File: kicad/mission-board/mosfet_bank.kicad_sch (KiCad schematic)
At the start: 28 parts, among them J10 MOSFET Ch2 Out, J11 MOSFET Ch3 Out, J12 MOSFET Ch4 Out, J9 MOSFET Ch1 Out, Q2 AO3400A, Q3 AO3400A, Q4 AO3400A, Q5 AO3400A, U4 INA180A2IDBVR, U5 INA180A2IDBVR, U6 INA180A2IDBVR, U7 INA180A2IDBVR

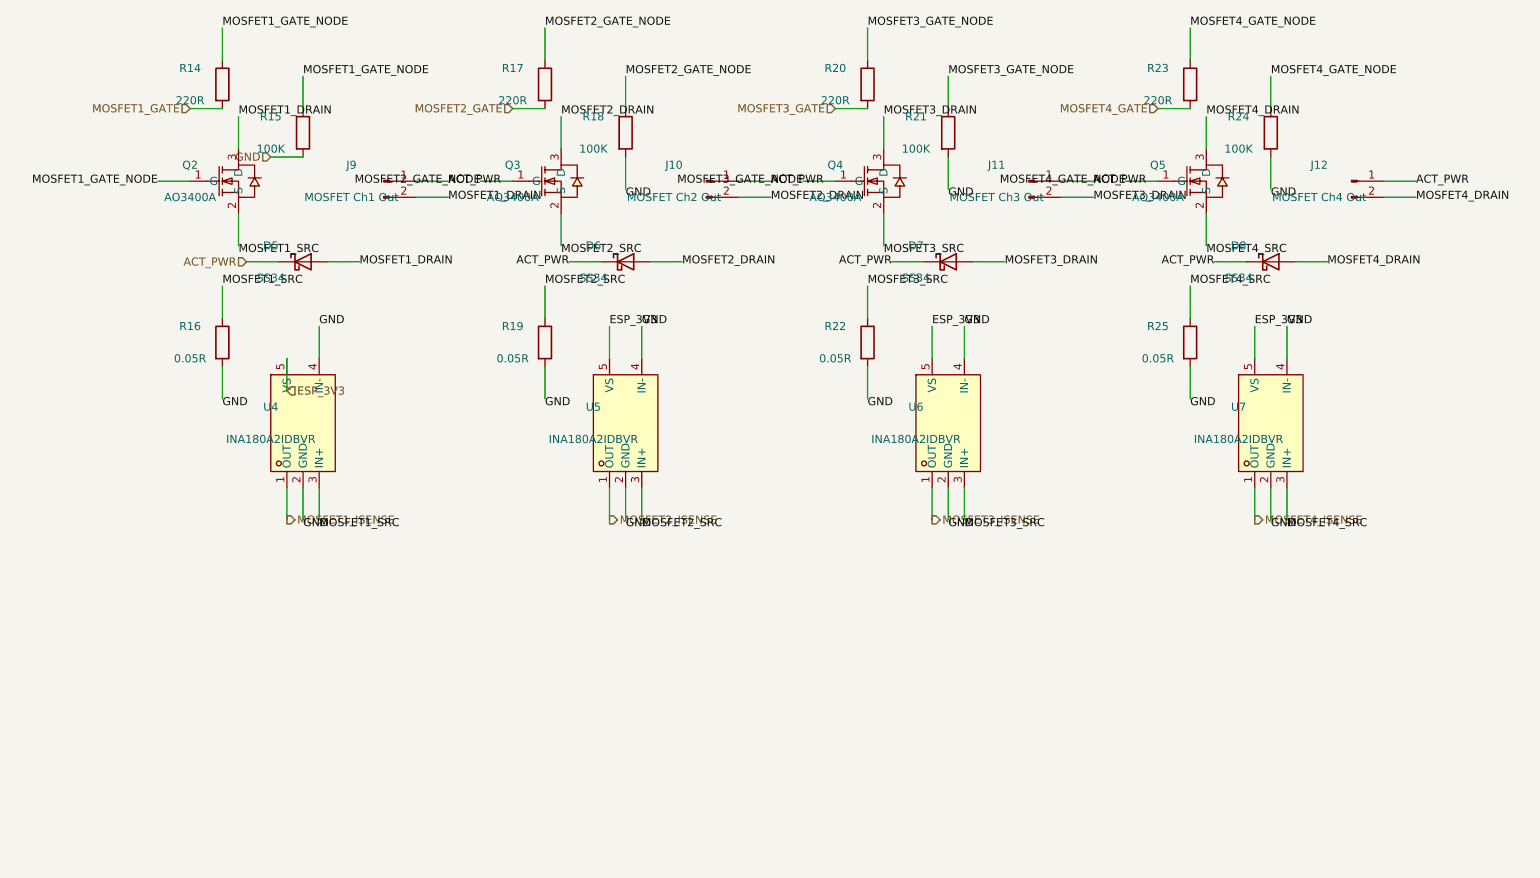
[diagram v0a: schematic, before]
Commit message: pcb progress
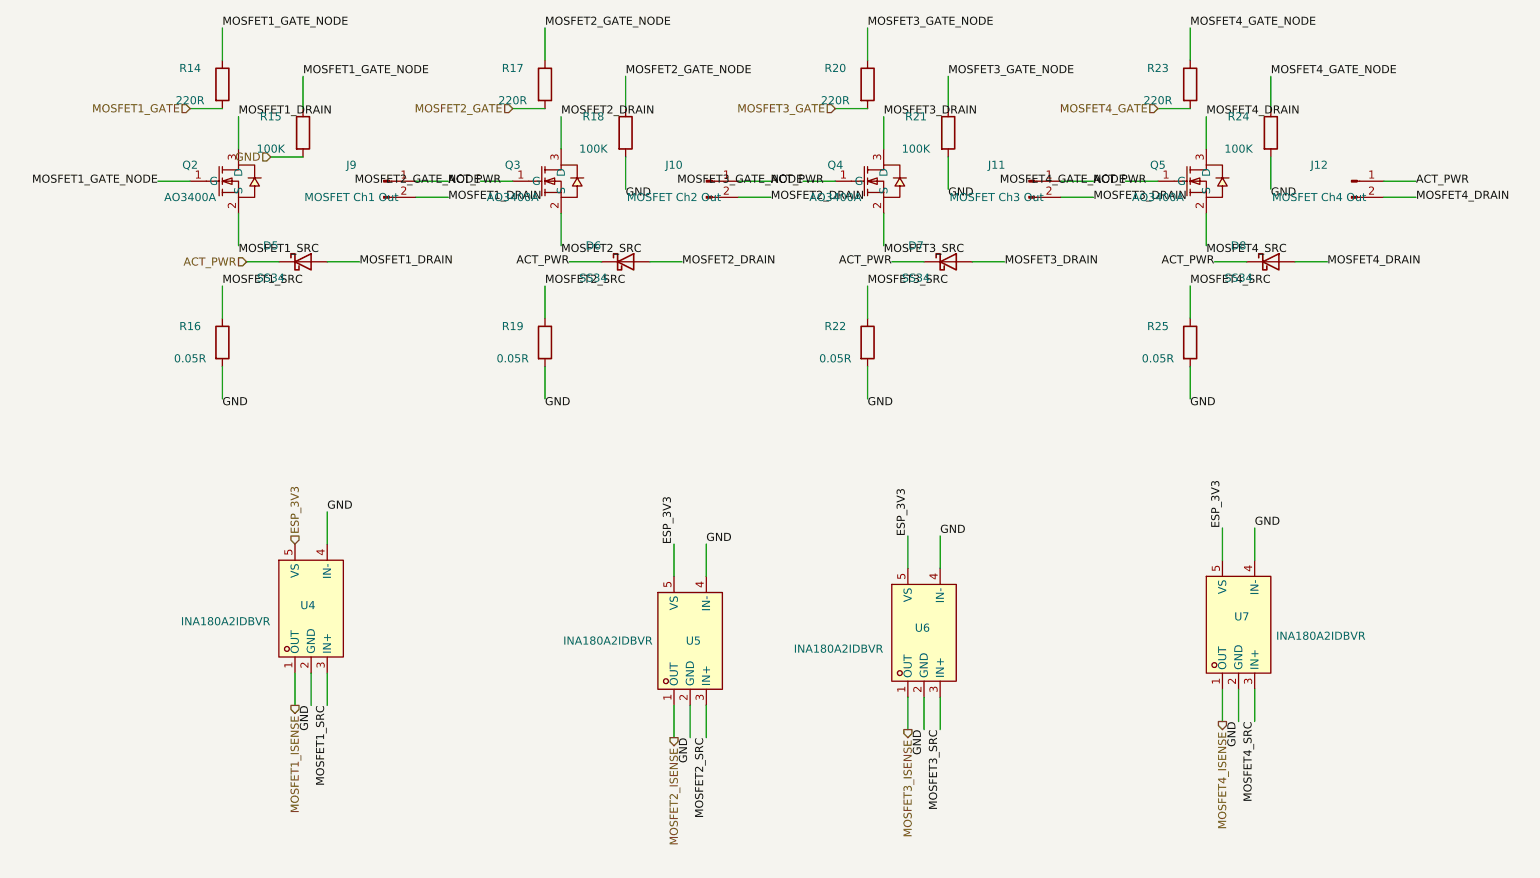
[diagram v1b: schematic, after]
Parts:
- J10, J11, J12, J9: footprint TerminalBlock_CUI:TerminalBlock_CUI_TB007-508-02_1x02_P5.08mm_Horizontal -> Connector_JST:JST_XH_B2B-XH-A_1x02_P2.50mm_Vertical
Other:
- moved on the sheet: U4, U5, U6, U7
